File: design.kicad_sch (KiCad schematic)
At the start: 14 parts, among them J1 Conn_01x02, J2 Conn_01x02, J3 Conn_01x03, J4 Conn_01x03, U1 TPS61099YFFT

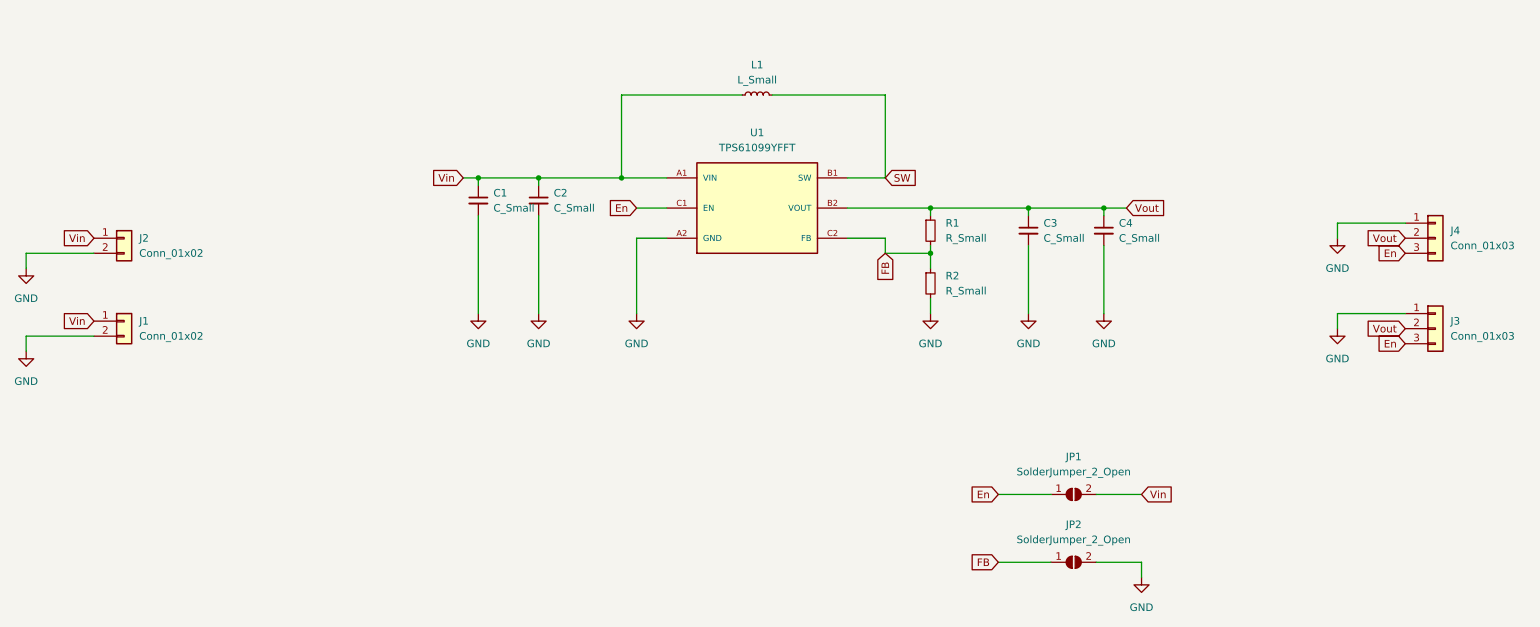
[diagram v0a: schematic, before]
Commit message: Update design.kicad_sch
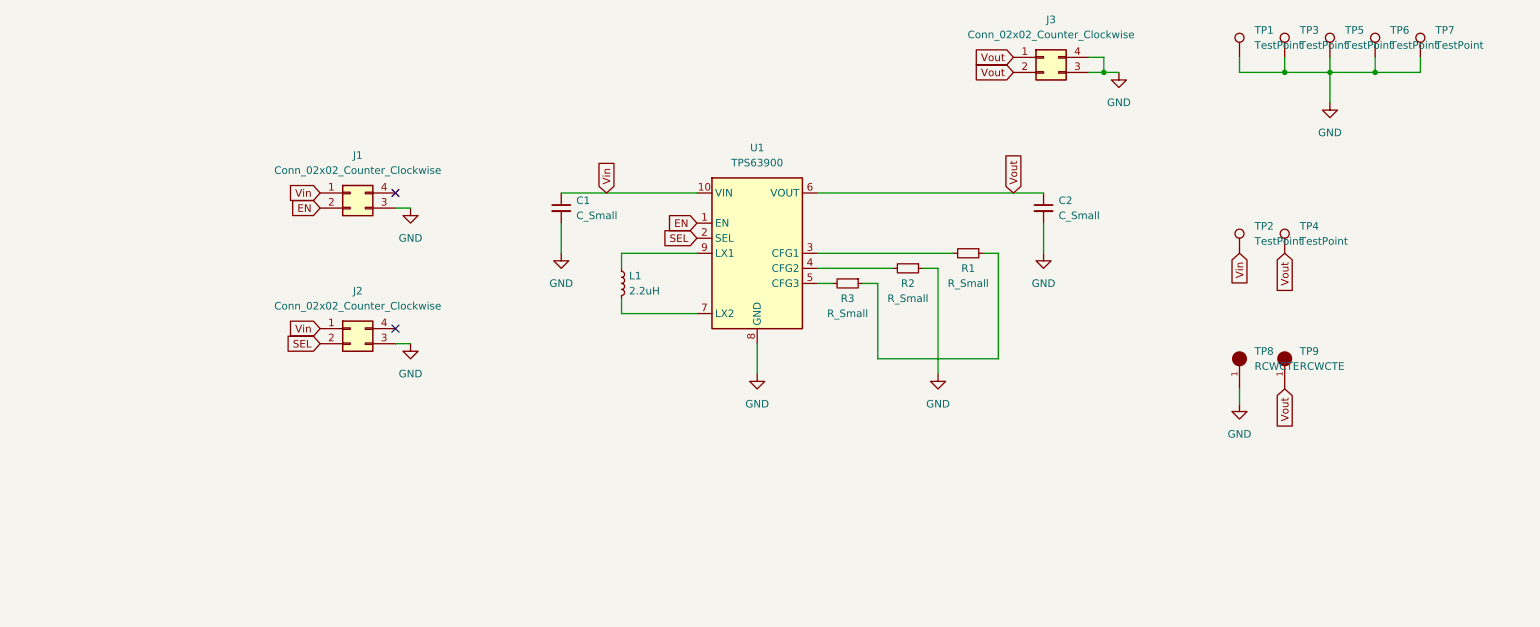
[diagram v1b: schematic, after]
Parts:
- removed C3, C4: C_Small, Capacitor_SMD:C_0805_2012Metric, symbol Device:C_Small
- removed J1, J2: Conn_01x02, Connector_PinHeader_2.54mm:PinHeader_1x02_P2.54mm_Vertical, symbol Connector_Generic:Conn_01x02
- removed J3, J4: Conn_01x03, Connector_PinHeader_2.54mm:PinHeader_1x03_P2.54mm_Vertical, symbol Connector_Generic:Conn_01x03
- removed JP1, JP2: SolderJumper_2_Open, Jumper:SolderJumper-2_P1.3mm_Open_RoundedPad1.0x1.5mm, symbol Jumper:SolderJumper_2_Open
- removed U1: TPS61099YFFT, Converter_DCDC_custom:BGA6N40P3X2_122X88X62N, symbol Converter_DCDC_custom:TPS61099YFFT
- added J1, J2, J3: Conn_02x02_Counter_Clockwise, Connector_PinSocket_2.54mm:PinSocket_2x02_P2.54mm_Vertical, symbol Connector_Generic:Conn_02x02_Counter_Clockwise
- added R3: R_Small, Resistor_SMD:R_0805_2012Metric, symbol Device:R_Small
- added TP1, TP2, TP3, TP4, TP5, TP6, TP7: TestPoint, TestPoint:TestPoint_Pad_D3.0mm, symbol Connector:TestPoint
- added TP8, TP9: RCWCTE, Snapeda:RCWCTE_TP420X150, symbol Snapeda:RCWCTE
- added U1: TPS63900, Package_SON:WSON-10-1EP_2.5x2.5mm_P0.5mm_EP1.2x2mm_ThermalVias, symbol Regulator_Switching:TPS63900
- C1, C2: footprint Capacitor_SMD:C_0805_2012Metric -> Capacitor_SMD:C_0603_1608Metric
- L1: value L_Small -> 2.2uH
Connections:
- net GND: now also R2.1, J1.3 (Pin_3), J2.3 (Pin_3), J3.3 (Pin_3), J3.4 (Pin_4), TP1.1, TP3.1, TP5.1, TP6.1, TP7.1, TP8.1, U1.11 (GND), U1.8 (GND); no longer R2.2
- net Vin: now also J1.1 (Pin_1), J2.1 (Pin_1), TP2.1, U1.10 (VIN); no longer C2.1, L1.1
- net Vout: now also C2.1, J3.1 (Pin_1), J3.2 (Pin_2), TP4.1, TP9.1, U1.6 (VOUT); no longer R1.1
- net FB: no longer names the net of R1.2
- net FB: now also U1.3 (CFG1); no longer R2.1
- net SW: no longer names the net of L1.2
- net SW: now also U1.7 (LX2)
- new net: R1.1, R3.1
- new net: R2.2, U1.4 (CFG2)
- new net: R3.2, U1.5 (CFG3)
- new net: L1.1, U1.9 (LX1)
- new net EN: J1.2 (Pin_2), U1.1 (EN)
- new net SEL: J2.2 (Pin_2), U1.2 (SEL)
- no-connect marks 0 -> 2
